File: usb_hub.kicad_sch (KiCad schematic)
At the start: 27 parts, among them J1 USB_C_Receptacle_USB2.0_16P, J2 Barrel_Jack_Switch, U1 USB2514B_Bi, U2 SPX3819M5-L, U3 USBLC6-2SC6

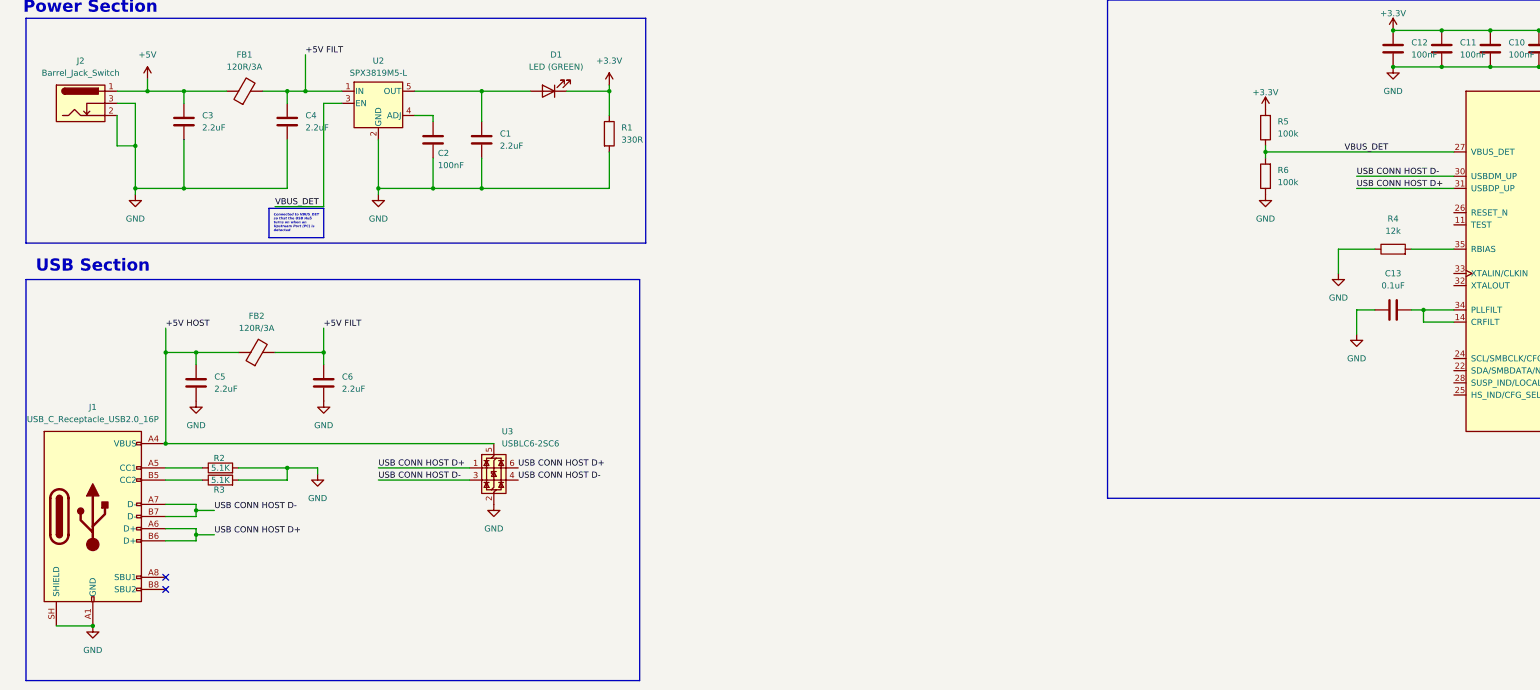
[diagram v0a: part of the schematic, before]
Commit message: Added modification to schematic
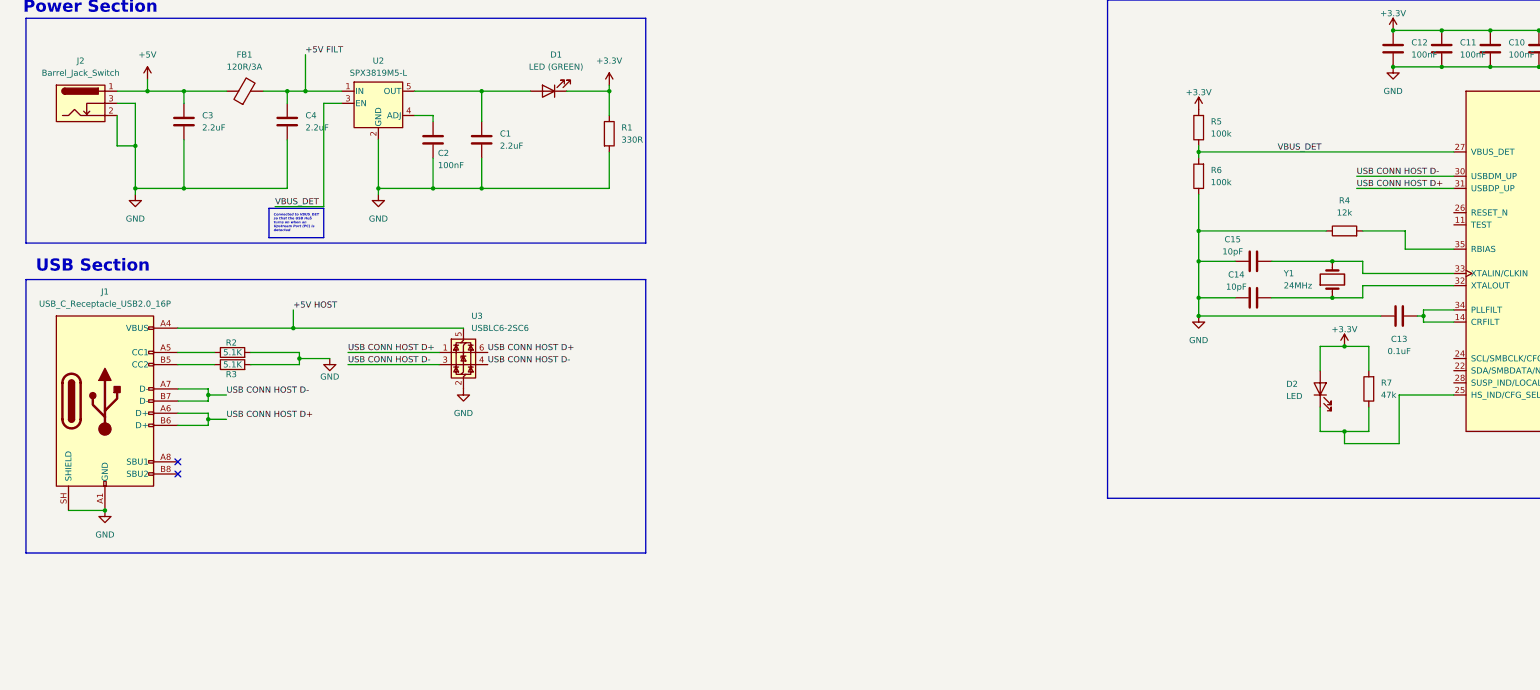
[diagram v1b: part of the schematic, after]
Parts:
- removed C5, C6: 2.2uF, symbol Device:C
- removed FB2: 120R/3A, symbol Device:FerriteBead
- added C14, C15: 10pF, symbol Device:C
- added D2: LED, symbol Device:LED
- added R7: 47k, symbol Device:R
- added Y1: 24MHz, symbol Device:Crystal
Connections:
- net +3.3V: now also D2.2 (A), R7.2
- net GND: now also C14.1, C15.1
- net at U1.25 (HS_IND/CFG_SEL1): now also D2.1 (K), R7.1
- net at U1.32 (XTALOUT): now also C14.2, Y1.1
- net at U1.33 (XTALIN/CLKIN): now also C15.2, Y1.2
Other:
- moved on the sheet: C13, J1, R2, R3, R4, R5, R6, U3
